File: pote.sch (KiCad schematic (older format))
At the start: 16 parts, among them J1 Conn_01x01, J2 Conn_01x01, J3 Conn_01x01, J4 Conn_01x01, J5 Conn_01x01, J6 Conn_01x01, J7 Conn_01x01, J8 Conn_01x01, U1 Opamp_Quad_Generic

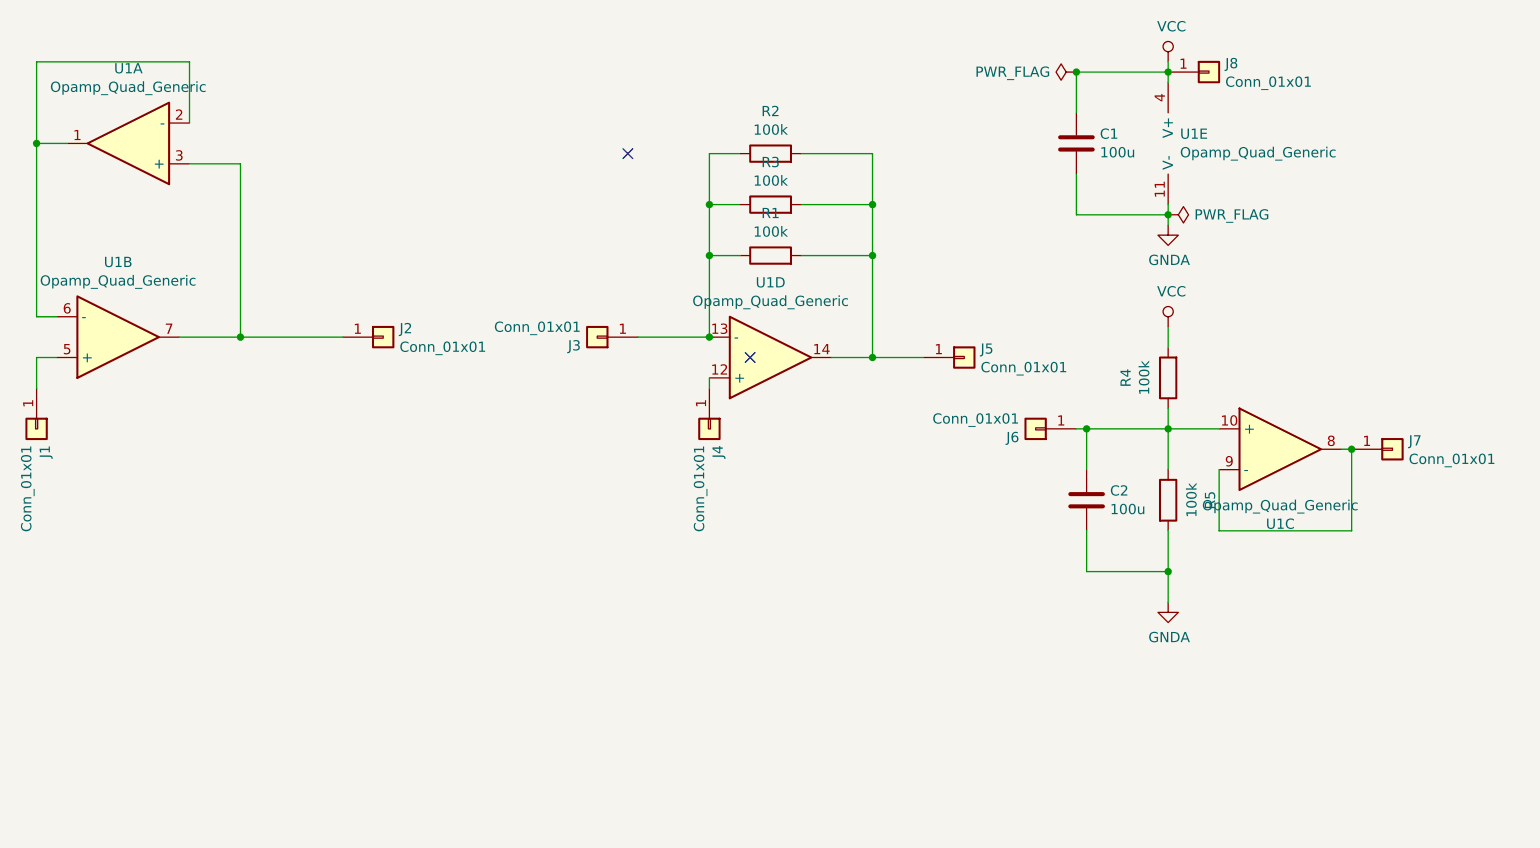
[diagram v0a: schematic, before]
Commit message: routing 1st cut
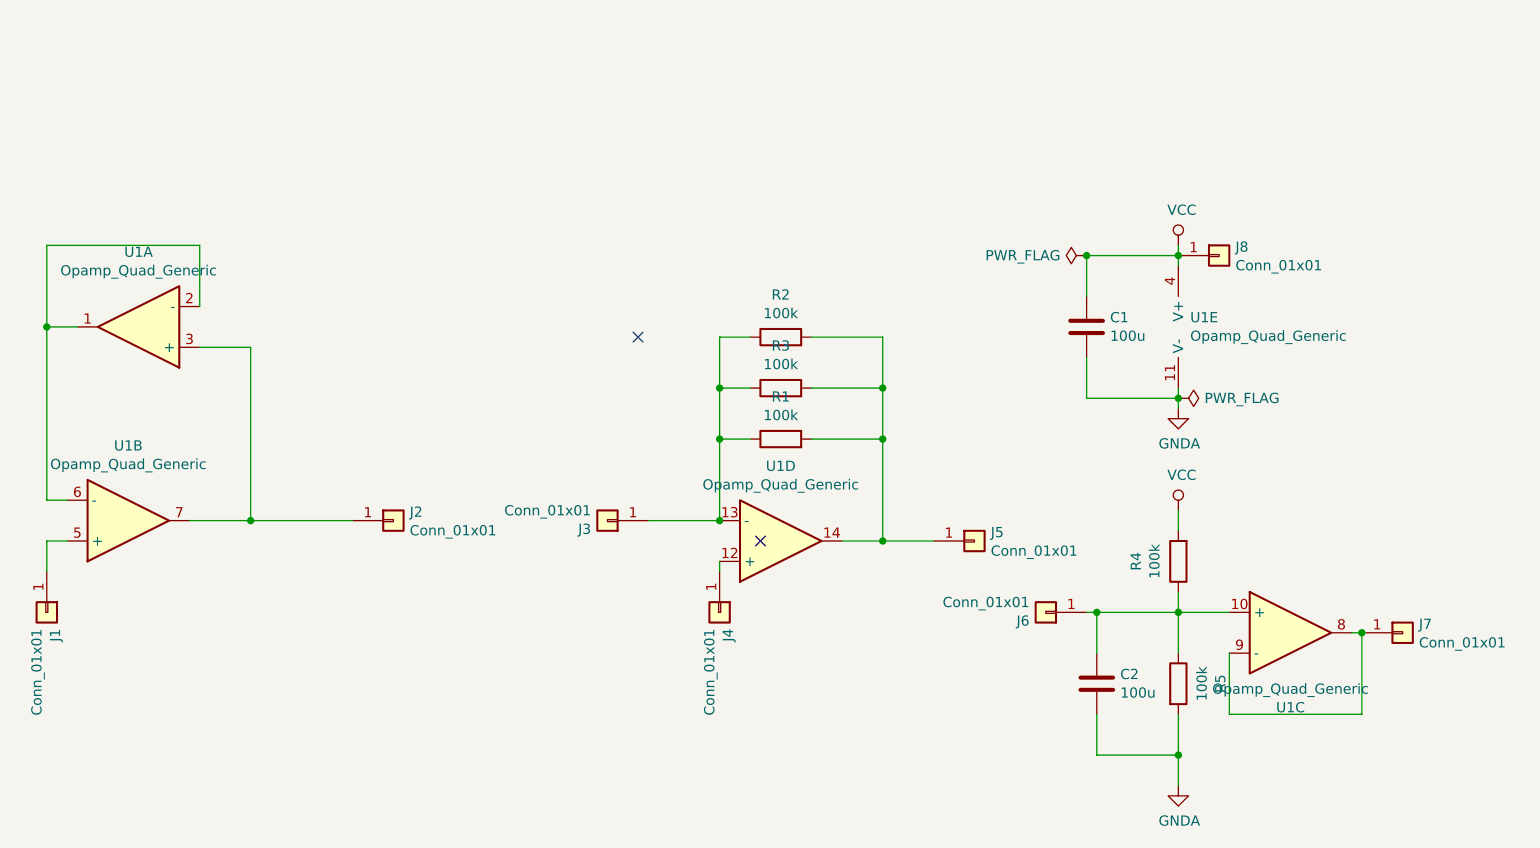
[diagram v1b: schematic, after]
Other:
- moved on the sheet: C1, C2, J1, J2, J3, J4, J5, J6, J7, J8, R1, R2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
